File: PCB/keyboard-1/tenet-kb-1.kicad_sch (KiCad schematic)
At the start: 114 parts, among them SW1 SW_Push, U1 ATmega32U4-A, Y1 16MHz

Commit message: footprints assigned
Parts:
- C1, C2, C3, C4, C5, C6, C7: footprint (none) -> Capacitor_SMD:C_0805_2012Metric
- D1, D10, D11, D12, D13, D14, D15, D16, D17, D18, D19, D2, D20, D21, D22, D23, D24, D25, D26, D27, D28, D29, D3, D30, D31, D32, D33, D34, D35, D36, D37, D38, D39, D4, D40, D41, D42, D43, D44, D45, D46, D47, D48, D49, D5, D50, D6, D7, D8, D9: footprint (none) -> Diode_SMD:D_SOD-123
- MX1, MX10, MX11, MX12, MX13, MX14, MX15, MX16, MX17, MX18, MX19, MX2, MX20, MX21, MX22, MX23, MX24, MX26, MX27, MX28, MX29, MX3, MX30, MX31, MX32, MX33, MX34, MX35, MX36, MX37, MX38, MX39, MX4, MX40, MX41, MX42, MX43, MX44, MX45, MX46, MX47, MX48, MX49, MX5, MX6, MX7, MX8, MX9: footprint (none) -> Kailh_Choc:KailhChoc-1U
- MX25, MX50: footprint (none) -> Kailh_Choc:KailhChoc-1.75U
- R1, R2, R3, R4: footprint (none) -> Resistor_SMD:R_0805_2012Metric
- SW1: footprint (none) -> random-keyboard-parts.pretty-master:SKQG-1155865
- Y1: footprint (none) -> Crystal:Crystal_SMD_3225-4Pin_3.2x2.5mm

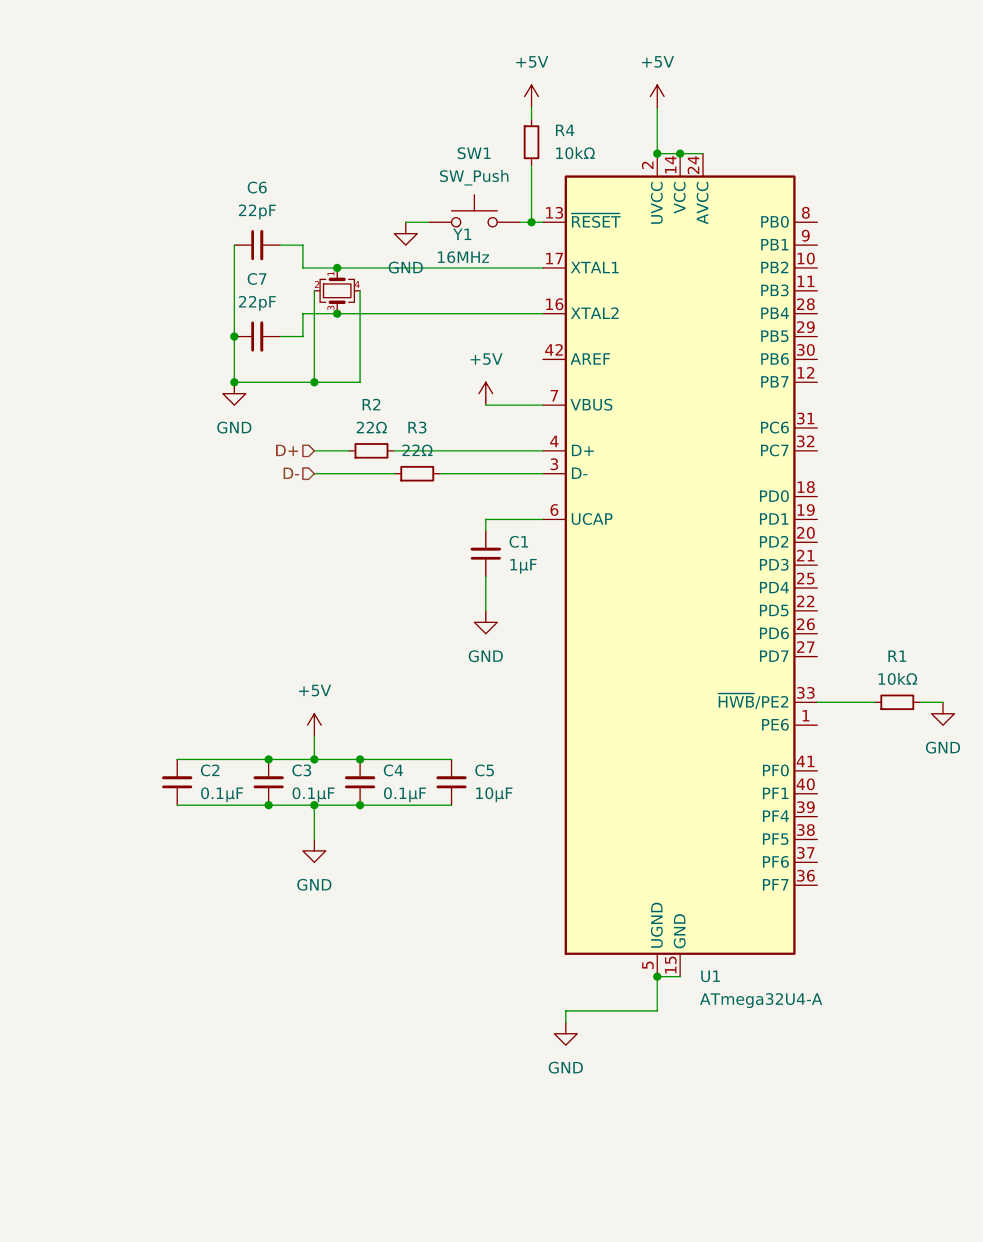
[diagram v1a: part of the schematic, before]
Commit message: pcb 1, mostly done
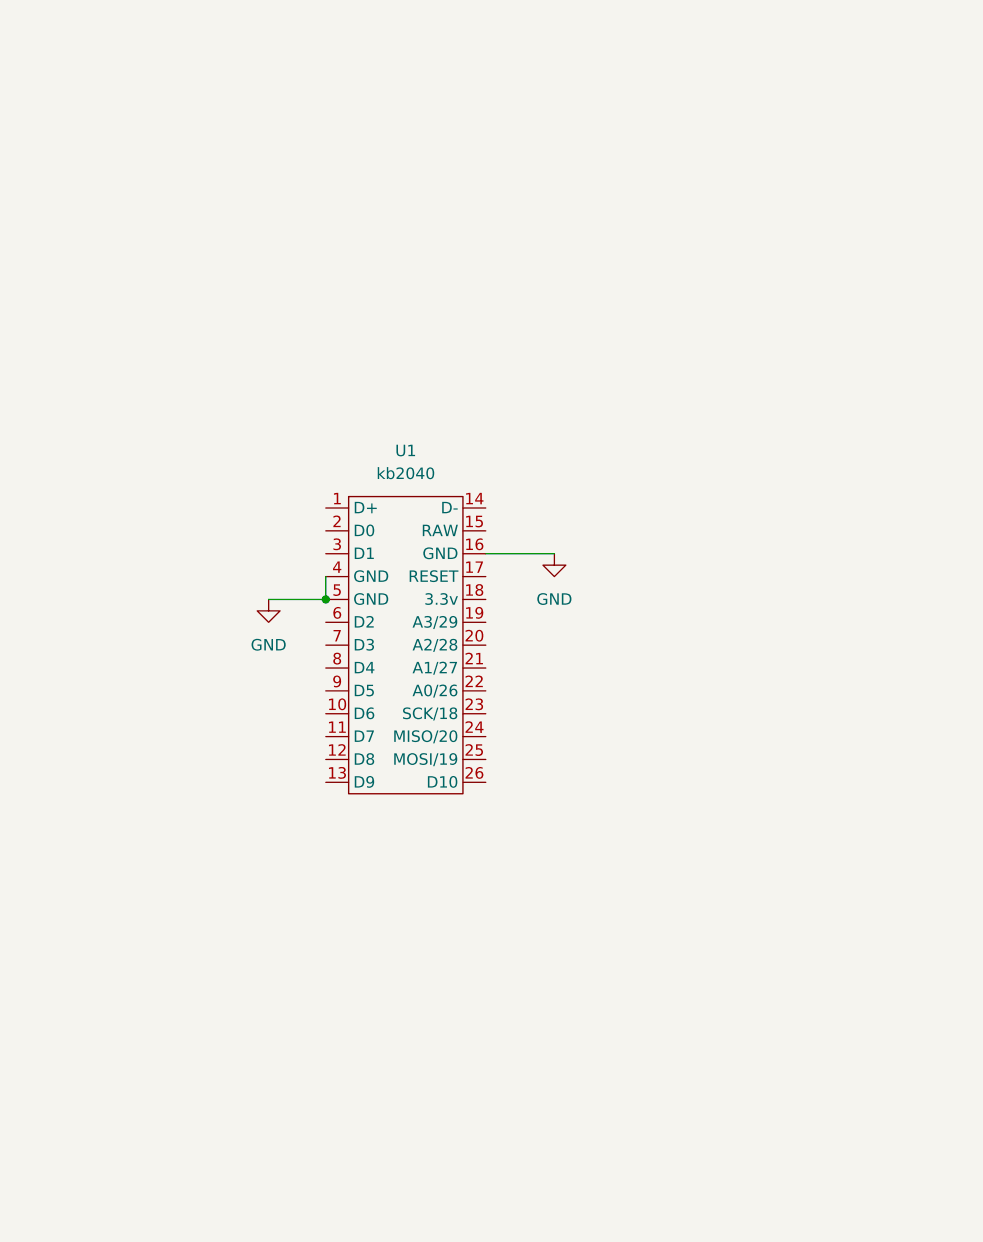
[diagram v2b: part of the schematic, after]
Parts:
- removed C1: 1µF, Capacitor_SMD:C_0805_2012Metric, symbol Device:C_Small
- removed C2, C3, C4: 0.1µF, Capacitor_SMD:C_0805_2012Metric, symbol Device:C_Small
- removed C5: 10µF, Capacitor_SMD:C_0805_2012Metric, symbol Device:C_Small
- removed C6, C7: 22pF, Capacitor_SMD:C_0805_2012Metric, symbol Device:C_Small
- removed R1, R4: 10kΩ, Resistor_SMD:R_0805_2012Metric, symbol Device:R_Small
- removed R2, R3: 22Ω, Resistor_SMD:R_0805_2012Metric, symbol Device:R_Small
- removed SW1: SW_Push, random-keyboard-parts.pretty-master:SKQG-1155865, symbol Switch:SW_Push
- removed U1: ATmega32U4-A, Package_QFP:TQFP-44_10x10mm_P0.8mm, symbol MCU_Microchip_ATmega:ATmega32U4-A
- removed Y1: 16MHz, Crystal:Crystal_SMD_3225-4Pin_3.2x2.5mm, symbol Device:Crystal_GND24_Small
- added U1: kb2040, kb2040:kb2040, symbol kb2040:kb2040
- MX1, MX10, MX11, MX12, MX13, MX14, MX15, MX16, MX17, MX18, MX19, MX2, MX20, MX21, MX22, MX23, MX24, MX26, MX27, MX28, MX29, MX3, MX30, MX31, MX32, MX33, MX34, MX35, MX36, MX37, MX38, MX39, MX4, MX40, MX41, MX42, MX43, MX44, MX45, MX46, MX47, MX48, MX49, MX5, MX6, MX7, MX8, MX9: footprint Kailh_Choc:KailhChoc-1U -> keyswitches.pretty-master:Kailh_socket_PG1350
- MX25, MX50: footprint Kailh_Choc:KailhChoc-1.75U -> keyswitches.pretty-master:Kailh_socket_PG1350
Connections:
- net GND: now also U1.16 (GND), U1.4 (GND), U1.5 (GND)
